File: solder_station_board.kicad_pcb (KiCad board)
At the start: 2 copper layers, 55.9 x 44.2 mm, 41 parts, among them J1 PWR_5_V, J2 INPUT, J3 RT_WELLER, J4 INPUT, J5 VFD_DISPLAY, J6 PWR_15V, J8 SERIAL, P1 ISP, Q1 IRF9540, Q2 2N7002, U4 TLC272, U5 LT1007, U6 ATMEGA168-20AU

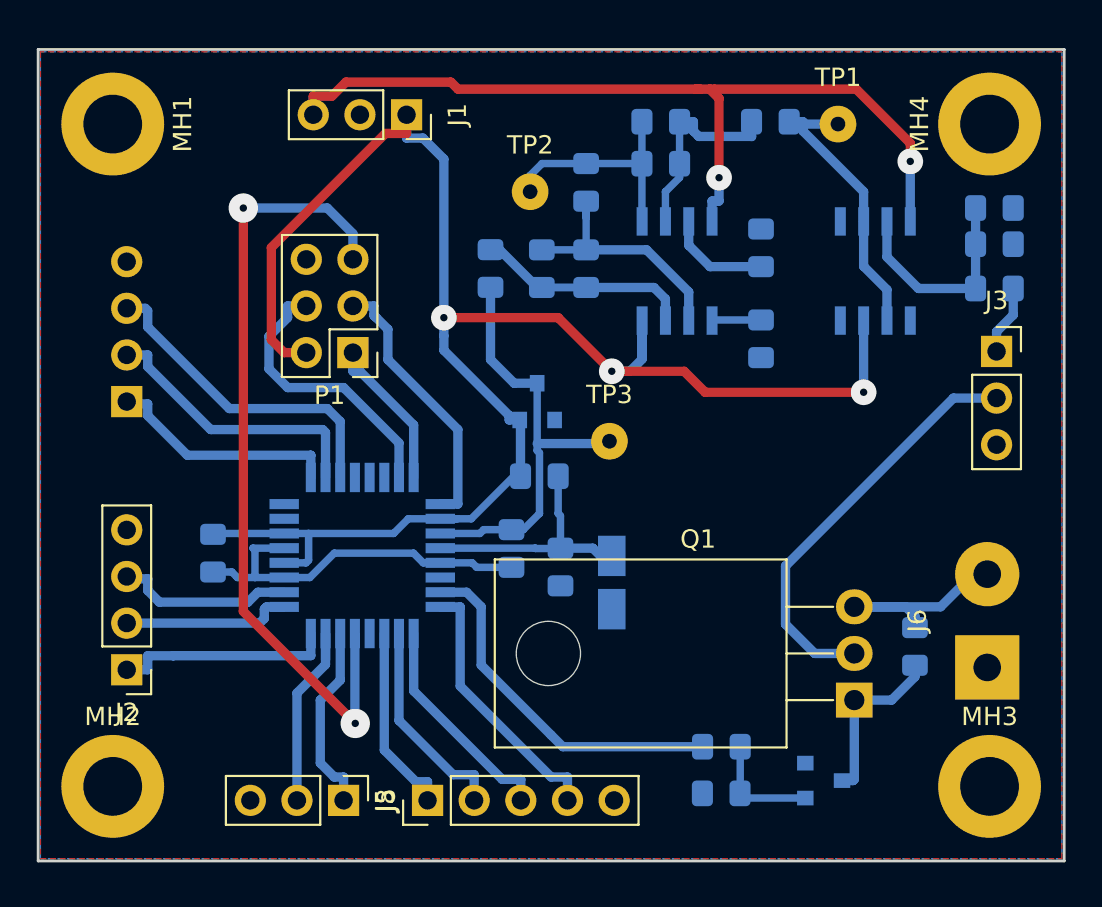
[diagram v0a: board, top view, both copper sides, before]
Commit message: small arrangements
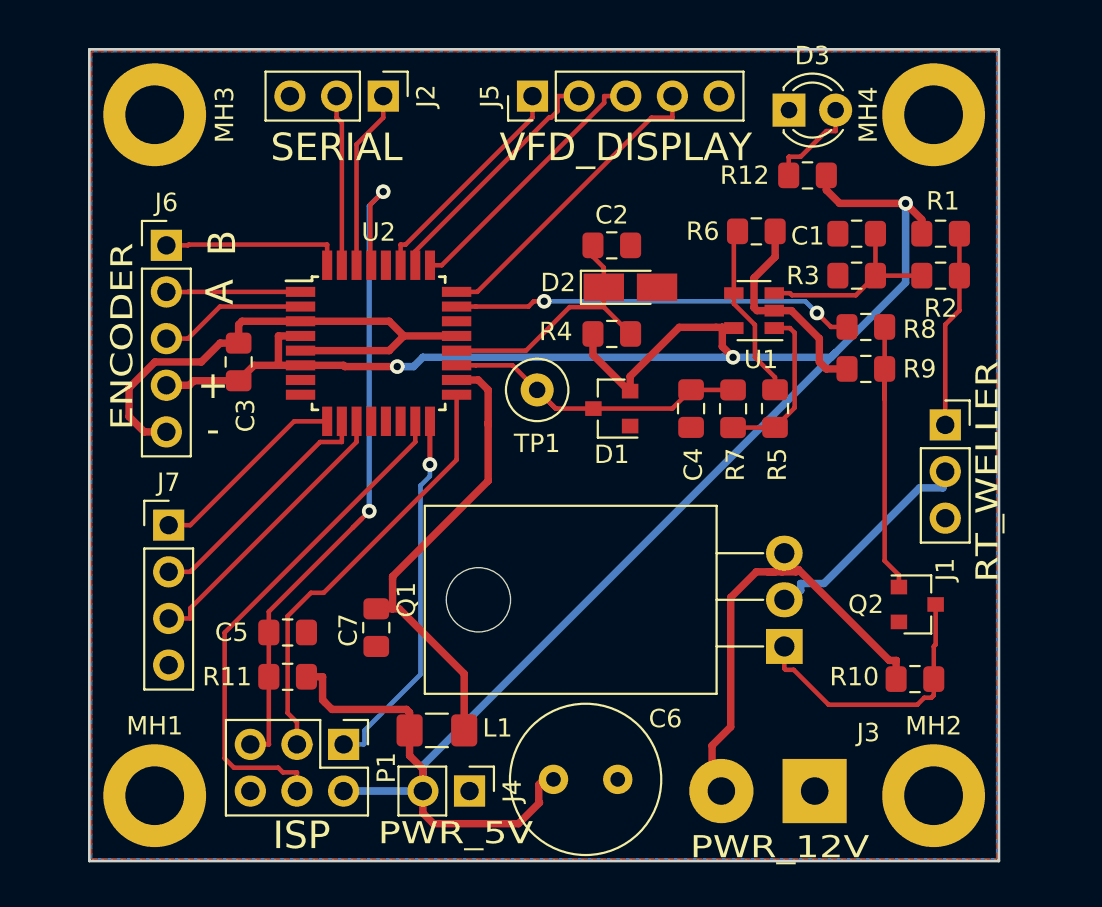
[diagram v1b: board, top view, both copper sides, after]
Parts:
- removed C13, C8, C9: 10n, Capacitor_SMD:C_0805_2012Metric_Pad1.15x1.40mm_HandSolder
- removed D8: 4V7, Diode_SMD:D_MicroMELF_Hadsoldering
- removed J8: SERIAL, Connector_PinHeader_2.54mm:PinHeader_1x03_P2.54mm_Vertical
- removed R13, R16: 1k, Resistor_SMD:R_0805_2012Metric_Pad1.15x1.40mm_HandSolder
- removed R14: 33k, Resistor_SMD:R_0805_2012Metric_Pad1.15x1.40mm_HandSolder
- removed R15: 10K, Resistor_SMD:R_0805_2012Metric_Pad1.15x1.40mm_HandSolder
- removed TP2, TP3: tp, Connector_Wire:SolderWirePad_1x01_Drill0.8mm
- removed U4: TLC272, Package_SO:SOIC-8_3.9x4.9mm_P1.27mm
- removed U5: LT1007, Package_SO:SOIC-8_3.9x4.9mm_P1.27mm
- removed U6: ATMEGA168-20AU, Package_QFP:TQFP-32_7x7mm_P0.8mm
- added C3: 10n, Capacitor_SMD:C_0805_2012Metric_Pad1.15x1.40mm_HandSolder, F.Cu at (53.8, 50.7)
- added C4: 10n, Capacitor_SMD:C_0805_2012Metric_Pad1.15x1.40mm_HandSolder, F.Cu at (78.4, 53.2)
- added C5: 100n, Capacitor_SMD:C_0805_2012Metric_Pad1.15x1.40mm_HandSolder, F.Cu at (56.5, 65.4)
- added C6: 100u, Capacitor_THT:C_Radial_D8.0mm_H7.0mm_P3.50mm, F.Cu at (71.0, 73.4)
- added D2: 4V7, Diode_SMD:D_MicroMELF_Hadsoldering, F.Cu at (75.1, 46.6)
- added D3: LED_G, LED_THT:LED_D3.0mm, F.Cu at (83.8, 37.0)
- added J7: INPUT, Connector_PinHeader_2.54mm:PinHeader_1x04_P2.54mm_Vertical, F.Cu at (50.0, 59.6)
- added L1: 10u, Inductor_SMD:L_1206_3216Metric_Pad1.42x1.75mm_HandSolder, F.Cu at (64.6, 70.8)
- added R1: 10M, Resistor_SMD:R_0805_2012Metric_Pad1.15x1.40mm_HandSolder, F.Cu at (92.0, 43.7)
- added R2: 5k6, Resistor_SMD:R_0805_2012Metric_Pad1.15x1.40mm_HandSolder, F.Cu at (92.0, 46.0)
- added R3: 100k, Resistor_SMD:R_0805_2012Metric_Pad1.15x1.40mm_HandSolder, F.Cu at (87.5, 46.0)
- added U1: OPA343, Package_TO_SOT_SMD:SOT-23-5, F.Cu at (81.9, 47.9)
- added U2: ATMEGA168-20AU, Package_QFP:TQFP-32_7x7mm_P0.8mm, F.Cu at (61.4, 49.7)
- C1, C2, D1, Q2, R11, R4: moved to F.Cu
- C7: value 10n -> 100n; moved to F.Cu
- J1: value PWR_5_V -> RT_WELLER
- J2: value INPUT -> SERIAL; footprint Connector_PinHeader_2.54mm:PinHeader_1x04_P2.54mm_Vertical -> Connector_PinHeader_2.54mm:PinHeader_1x03_P2.54mm_Vertical
- J3: value RT_WELLER -> PWR_15V; footprint Connector_PinSocket_2.54mm:PinSocket_1x03_P2.54mm_Vertical -> Connector_Wire:SolderWirePad_1x02_P5.08mm_Drill1.5mm
- J4: value INPUT -> PWR_5V; footprint Connector_PinHeader_2.54mm:PinHeader_1x04_P2.54mm_Vertical -> Connector_PinHeader_2.54mm:PinHeader_1x02_P2.54mm_Vertical; moved to F.Cu
- J6: value PWR_15V -> ENCODER; footprint Connector_Wire:SolderWirePad_1x02_P5.08mm_Drill1.5mm -> Connector_PinHeader_2.54mm:PinHeader_1x05_P2.54mm_Vertical
- MH1, MH2, MH3, MH4: value MP -> MH_Pad
- R10: value 1k -> 4k7; moved to F.Cu
- R12: value 22k -> 648; moved to F.Cu
- R5: value 5k6 -> 68k; moved to F.Cu
- R6: value 4k7 -> 100; moved to F.Cu
- R7: value 100k -> 5k6; moved to F.Cu
- R8: value 2k2 -> 1k; moved to F.Cu
- R9: value 1k -> 2k2; moved to F.Cu
- TP1: value tp -> TEMP; footprint Connector_Wire:SolderWirePad_1x01_Drill0.8mm -> TestPoint:TestPoint_Loop_D2.60mm_Drill0.9mm_Beaded
- moved MH3 58.4 mm to (49.2, 37.2)
- moved J6 50.3 mm to (49.9, 44.3), turned to 0 degrees
- moved MH2 44.7 mm to (91.7, 74.3)
- moved C7 40.7 mm to (61.3, 65.2), turned to 270 degrees
- moved J5 38.8 mm to (69.8, 36.2)
- moved MH1 36.6 mm to (49.2, 74.3)
- moved J2 34.2 mm to (61.7, 36.2), turned to 270 degrees
- moved J1 33.9 mm to (92.3, 54.1), turned to 0 degrees
- moved R10 31.4 mm to (90.6, 68.0), turned to 0 degrees
- moved J4 28.3 mm to (66.4, 74.1), turned to 270 degrees
- moved R8 26.6 mm to (88.0, 48.8)
- moved J3 25.9 mm to (85.2, 74.1), turned to 180 degrees
- moved R6 24.2 mm to (82.0, 43.6), turned to 0 degrees
- moved R9 22.0 mm to (88.0, 51.1)
- moved TP1 21.9 mm to (70.1, 52.2)
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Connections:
- C1 pad 2: Net-(C1-Pad2) -> GND
- C2 pad 2: Net-(C2-Pad2) -> GND
- J1 pad 1: +5V -> Net-(J1-Pad1)
- J1 pad 2: GND -> Net-(J1-Pad2)
- J1 pad 3: -5V -> GND
- J2 pad 1: /INP1 -> /RX
- J2 pad 2: /INP2 -> /TX
- J2 pad 3: /INP3 -> GND
- J3 pad 1: Net-(J3-Pad1) -> GND
- J3 pad 2: Net-(J3-Pad2) -> +15V
- J4 pad 1: /INP4 -> GND
- J4 pad 2: /INP5 -> +5V
- J6 pad 1: GND -> /INP1
- J6 pad 2: +15V -> /INP2
- Q1 pad 2: Net-(J3-Pad2) -> Net-(J1-Pad2)
- R10 pad 1: Net-(R10-Pad1) -> +15V
- R10 pad 2: Net-(C1-Pad1) -> Net-(Q1-Pad1)
- R11 pad 2: Net-(C8-Pad1) -> /RST
- R12 pad 1: Net-(C1-Pad1) -> Net-(D3-Pad2)
- R12 pad 2: Net-(C1-Pad2) -> +5V
- R4 pad 1: Net-(R4-Pad1) -> +5V
- R4 pad 2: GND -> Net-(C2-Pad1)
- R5 pad 1: Net-(C7-Pad1) -> Net-(R5-Pad1)
- R5 pad 2: Net-(J3-Pad1) -> Net-(R5-Pad2)
- R6 pad 1: +15V -> Net-(R5-Pad2)
- R6 pad 2: Net-(Q1-Pad1) -> GND
- R7 pad 1: GND -> /TEMP
- R7 pad 2: Net-(C7-Pad1) -> Net-(R5-Pad1)
- R8 pad 1: GND -> /SOLDER
- R9 pad 1: /SOLDER -> GND
- TP1 pad 1: Net-(R10-Pad1) -> /TEMP
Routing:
- net -5V: track 48.5 -> 0.00 mm, vias 2 -> 0
- net +5V: track 99.9 -> 130.0 mm
- net Net-(J3-Pad2): track 22.9 -> 0.00 mm
- net GND: track 20.5 -> 42.0 mm
- net Net-(C7-Pad1): track 11.9 -> 28.0 mm
- net Net-(R10-Pad1): track 15.4 -> 0.00 mm
- net +15V: track 12.1 -> 26.4 mm
- net Net-(C2-Pad2): track 14.2 -> 0.00 mm
- net /MISO: track 8.39 -> 22.3 mm, vias 0 -> 1
- net Net-(C8-Pad1): track 13.9 -> 0.00 mm
- net /MOSI: track 15.5 -> 28.3 mm
- net Net-(C1-Pad2): track 12.7 -> 0.00 mm
- net /RST: track 43.4 -> 56.0 mm
- net Net-(J1-Pad2): track 0.00 -> 12.3 mm
- net Net-(J8-Pad2): track 11.2 -> 0.00 mm
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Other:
- board size 55.9 x 44.2 mm -> 49.5 x 44.2 mm
- net class power added: clearance 0.2, trace_width 0.4064, via_dia 0.8, via_drill 0.4
- board text added: "+"
- board text added: "-"
- board text added: "A"
- board text added: "B"
- board text added: "ENCODER"
- board text added: "ISP"
- board text added: "PWR_12V"
- board text added: "PWR_5V"
- board text added: "RT_WELLER"
- board text added: "SERIAL"
- board text added: "VFD_DISPLAY"
